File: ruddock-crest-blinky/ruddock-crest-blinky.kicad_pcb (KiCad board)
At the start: 2 copper layers, 38.1 x 45.7 mm, 33 parts, among them Q1 IRFML8244, SW1 JS202011JCQN, SW2 PTS526 SK15 SMTR2 LFS, U1 ATtiny85-20SU, U2 74HC595

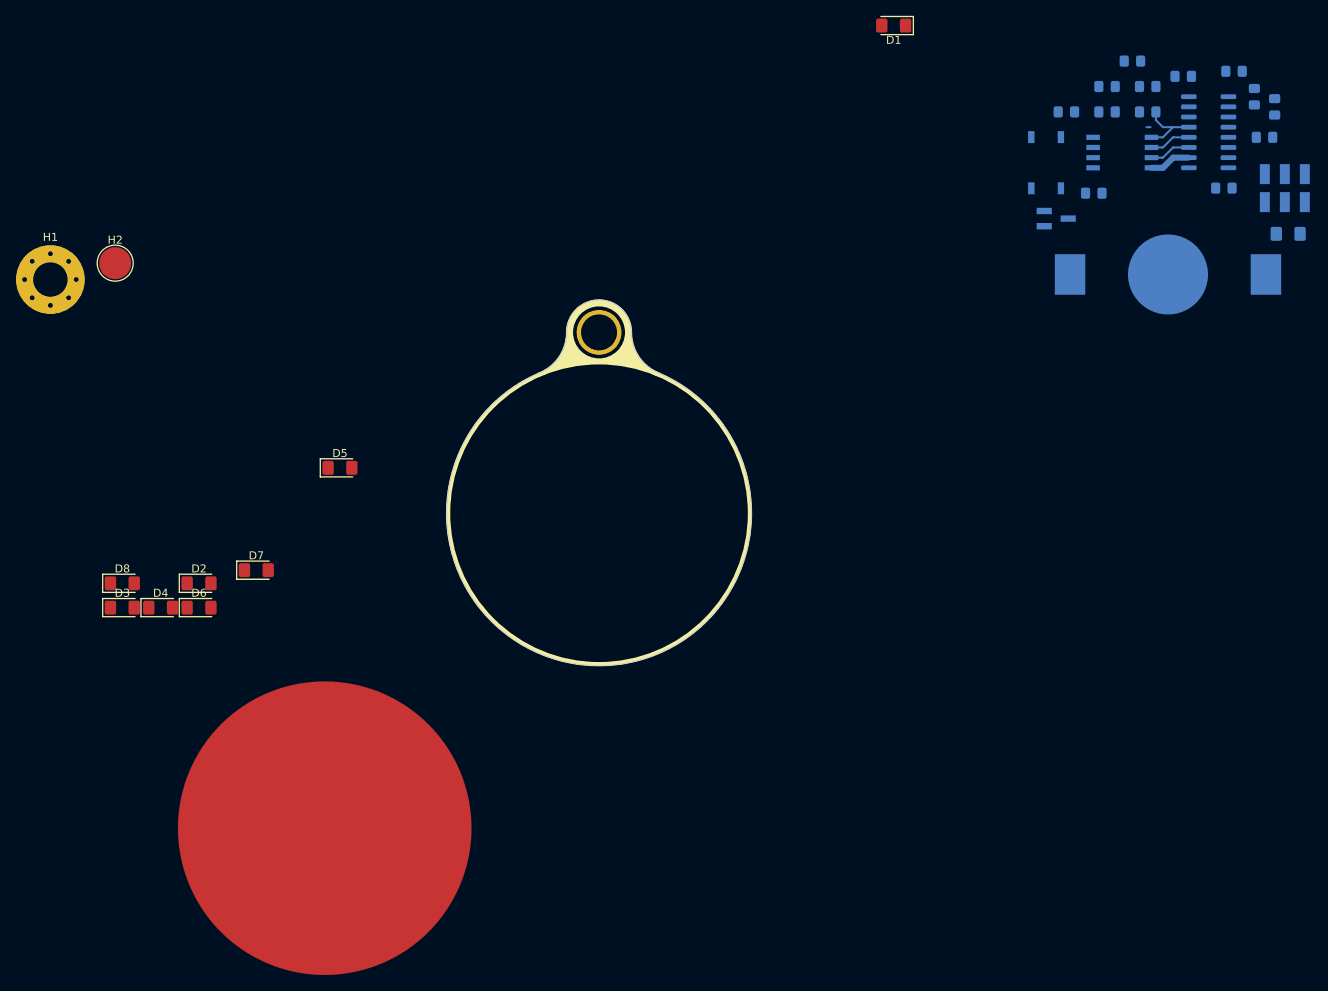
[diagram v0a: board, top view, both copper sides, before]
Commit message: Finish placement
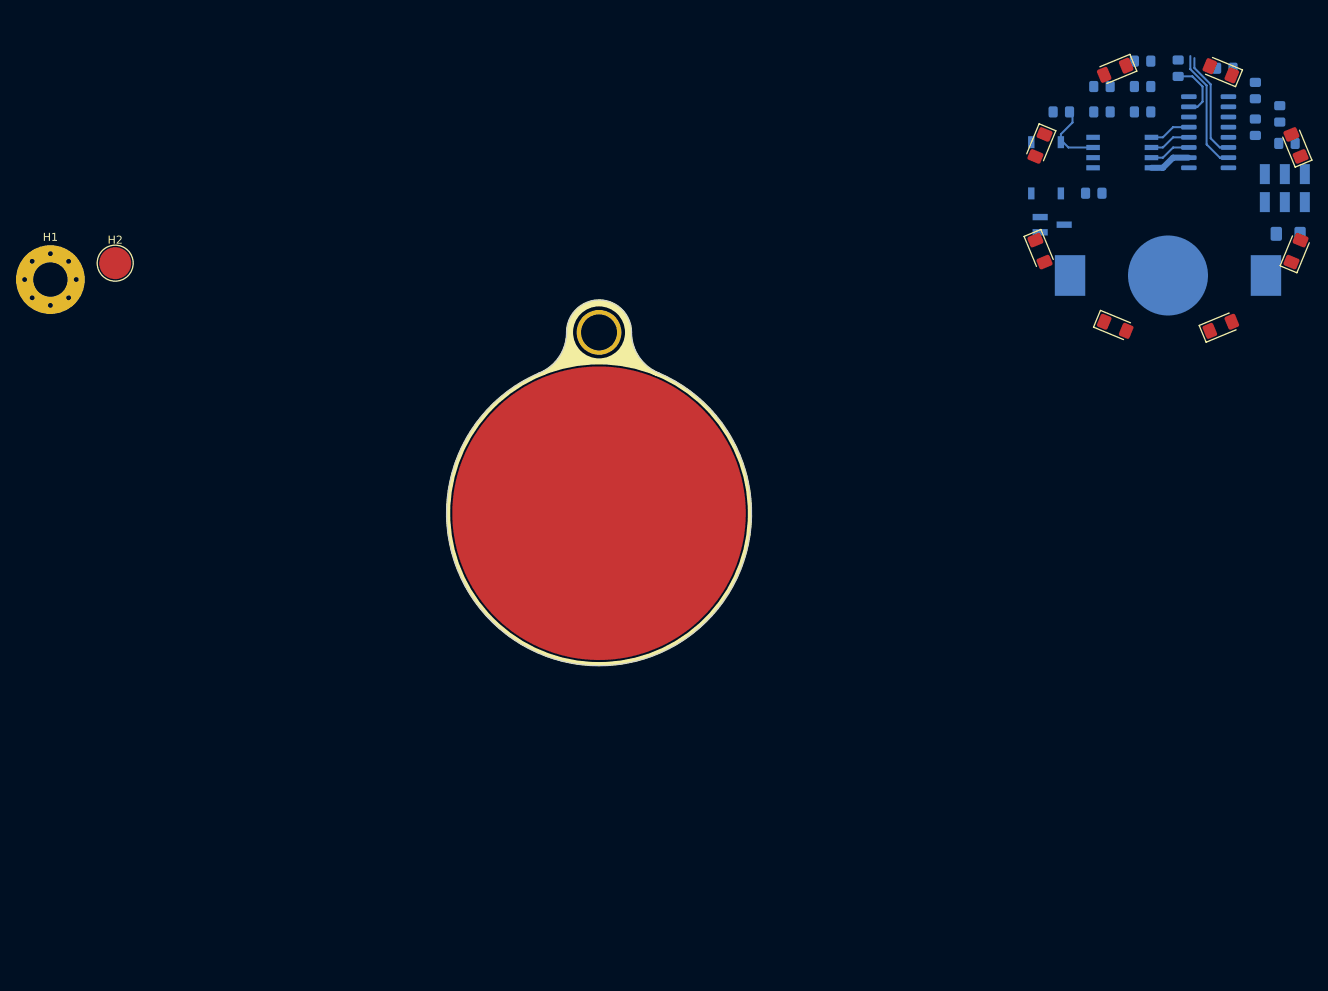
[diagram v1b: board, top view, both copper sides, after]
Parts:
- moved D3 153.3 mm to (228.1, 75.2), turned to 67.5 degrees
- moved D2 147.6 mm to (228.1, 62.0), turned to 112.5 degrees
- moved D8 139.7 mm to (205.5, 52.6), turned to 202.5 degrees
- moved D4 137.1 mm to (218.7, 84.6), turned to 22.5 degrees
- moved D6 114.2 mm to (196.1, 75.2), turned to 292.5 degrees
- moved D7 111.4 mm to (196.1, 62.0), turned to 247.5 degrees
- moved D5 98.5 mm to (205.5, 84.6), turned to 337.5 degrees
- moved G*** 52.2 mm to (141.0, 108.0)
- moved G*** 43.2 mm to (141.0, 108.0)
- moved D1 41.3 mm to (218.7, 52.6), turned to 157.5 degrees
- moved R6 9.66 mm to (227.0, 61.7), turned to 0 degrees
- moved R8 3.42 mm to (208.9, 54.6)
- moved R7 3.24 mm to (208.9, 51.4)
- moved R5 1.70 mm to (223.0, 59.7), turned to 270 degrees
- moved R2 1.21 mm to (219.2, 52.3)
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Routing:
- net /LED8: track 0.00 -> 15.3 mm
- net /LED7: track 0.00 -> 13.6 mm
- net /USER: track 0.00 -> 9.03 mm
- net /LED1: track 0.00 -> 7.45 mm
- net /~OE: track 9.20 -> 5.13 mm
- net /LED4: track 0.00 -> 0.83 mm
